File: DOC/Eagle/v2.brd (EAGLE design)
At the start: 55 x 55 mm, 18 parts, among them M1 RF-LORA-868-SO, X1 SMA-142-0701-871/876

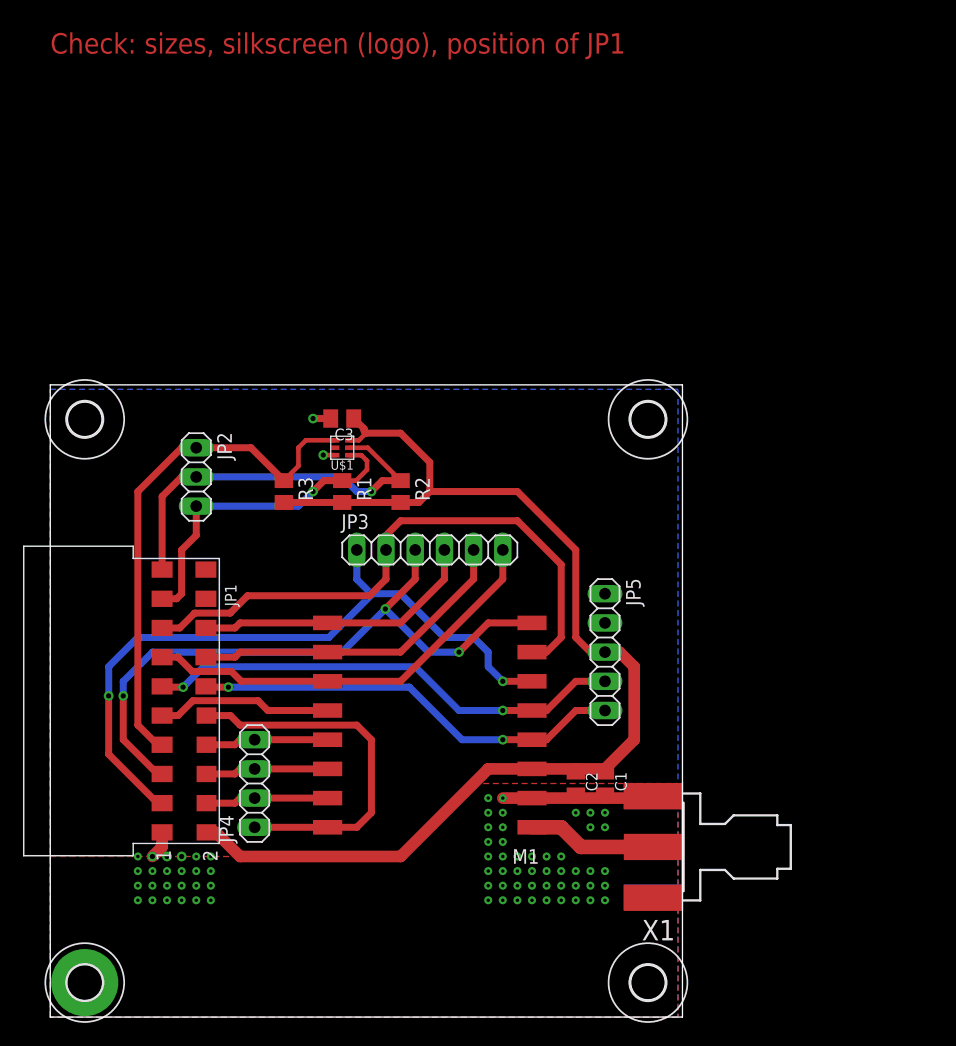
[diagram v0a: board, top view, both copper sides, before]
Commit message: Updated board design
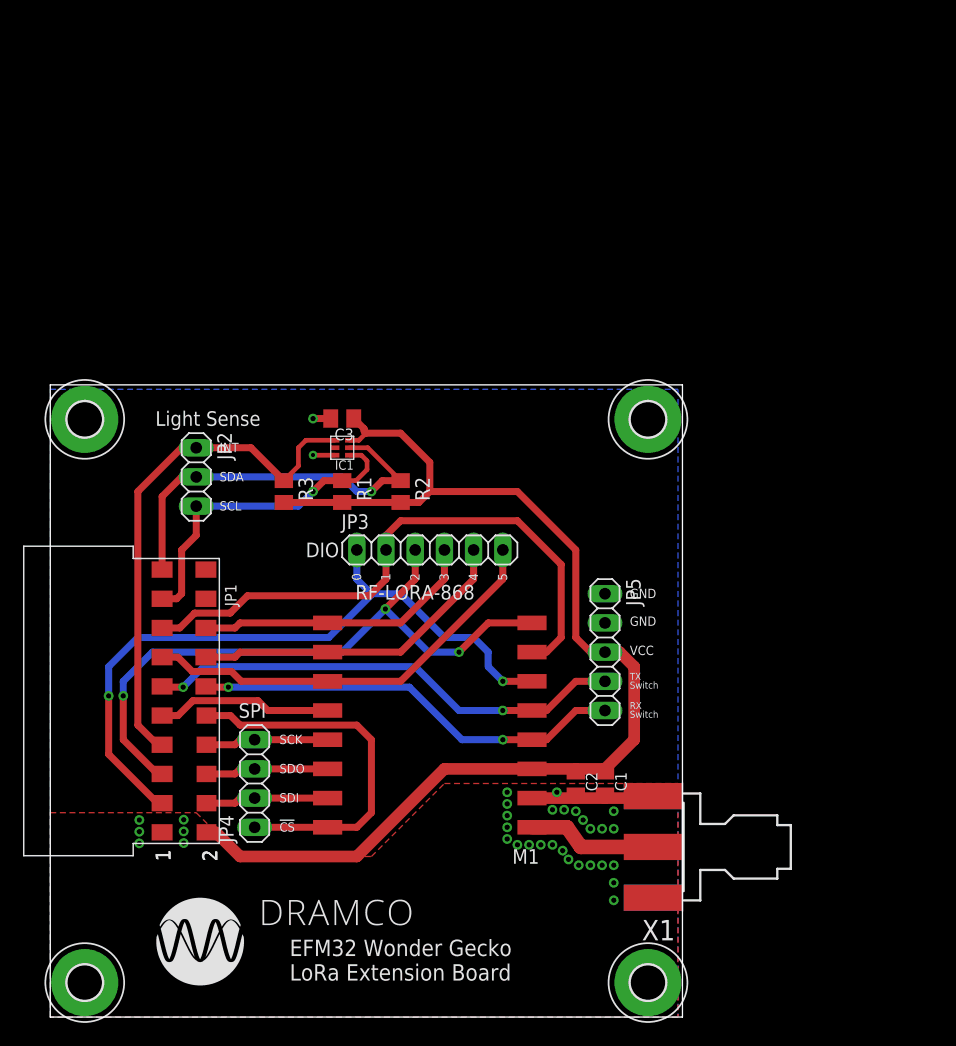
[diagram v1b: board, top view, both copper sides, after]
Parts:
- H1, H2, H3: value MOUNT-HOLE3.0 -> MOUNT-PAD-ROUND3.0; device holes:3,0 -> holes:3,0-PAD
- moved H1 49.0 mm to (52.0, 52.0)
- moved H3 49.0 mm to (52.0, 3.00)
- renumbered U$1 to IC1
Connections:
- net GND: now also H1.B3,0, H2.B3,0, H3.B3,0
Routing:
- net GND: track 18.7 -> 14.6 mm, vias 42 -> 34
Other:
- board text added: "!CS"
- board text added: "0"
- board text added: "1"
- board text added: "2"
- board text added: "3"
- board text added: "4"
- board text added: "5"
- board text added: "DIO"
- board text added: "DRAMCO research group"
- board text added: "Design by:"
- board text added: "EFM32 Wonder Gecko"
- board text added: "EFM32 Wonder Gecko LoRa Extension Board"
- board text added: "GND"
- board text added: "Geoffrey Ottoy & Gilles Callebaut"
- board text added: "INT"
- board text added: "KU Leuven - Technology Campus Ghent"
- board text added: "Light Sense"
- board text added: "LoRa Extension Board (v2.0)"
- board text added: "RF-LORA-868"
- board text added: "RX"
- board text added: "SCK"
- board text added: "SCL"
- board text added: "SDA"
- board text added: "SDI"
- board text added: "SDO"
- board text added: "SPI"
- board text added: "Switch"
- board text added: "TX"
- board text added: "VCC"
- board text removed: "Check: sizes!, silkscreen (logo), position of JP1"

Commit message: Final touches to board design, Gerber files
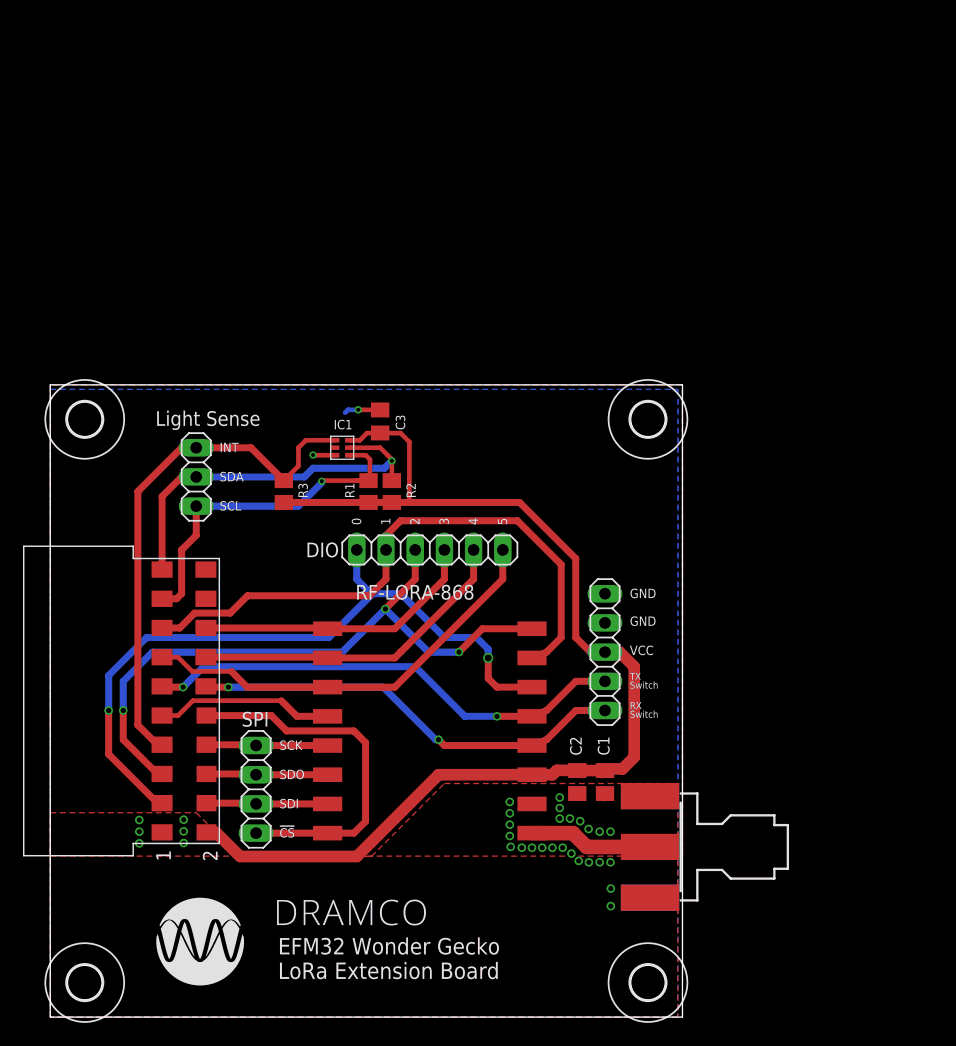
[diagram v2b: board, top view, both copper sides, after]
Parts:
- H1, H2, H3, H4: value MOUNT-PAD-ROUND3.0 -> MOUNT-HOLE3.0; device holes:3,0-PAD -> holes:3,0
- moved H1 69.3 mm to (3.00, 3.00)
- moved H2 69.3 mm to (52.0, 3.00)
- moved H3 49.0 mm to (52.0, 52.0)
- moved H4 49.0 mm to (3.00, 52.0)
- moved C3 3.31 mm to (28.7, 51.8), turned to 90 degrees
- moved R1 2.29 mm to (27.7, 45.7)
- moved R2 0.76 mm to (29.7, 45.7)
- moved JP4 0.52 mm to (17.9, 19.8)
- moved M1 0.51 mm to (33.0, 24.9)
- moved X1 0.25 mm to (54.7, 14.8)
- moved C2 0.18 mm to (45.8, 20.4)
- moved C1 0.13 mm to (48.3, 20.4)
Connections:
- net GND: no longer H1.B3,0, H2.B3,0, H3.B3,0, H4.B3,0
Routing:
- net GND: track 14.6 -> 5.44 mm, vias 34 -> 33
- net LIGHT_SENSE_SCL: track 28.7 -> 30.9 mm
- net VCC: track 103.5 -> 105.3 mm
- net LIGHT_SENSE_SDA: track 34.3 -> 33.6 mm
- net ANT: track 11.4 -> 10.8 mm
- net !CS: track 32.3 -> 31.6 mm
- net DIO0: track 61.8 -> 62.4 mm
- added copper zone on layer 1, net TEST
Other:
- board text added: "Designed by: Geoffrey Ottoy, Gilles Callebaut, Guus Leenders"
- board text removed: "Design by:"
- board text removed: "Geoffrey Ottoy & Gilles Callebaut"
